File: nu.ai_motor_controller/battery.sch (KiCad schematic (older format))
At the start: 42 parts, among them J12 XT60_RA_MALE, J13 S4B-XH-A, J14 NP_Screw_Terminal_01x02, J15 XT60_RA_MALE, J16 S4B-XH-A, J17 S4B-XH-A, J18 XT60_RA_FEMALE, Q1 IRF9540N, Q2 SSM3K35AMFV, Q4 SSM3K35AMFV, SW2 TACTILE_SWITCH, SW3 TACTILE_SWITCH

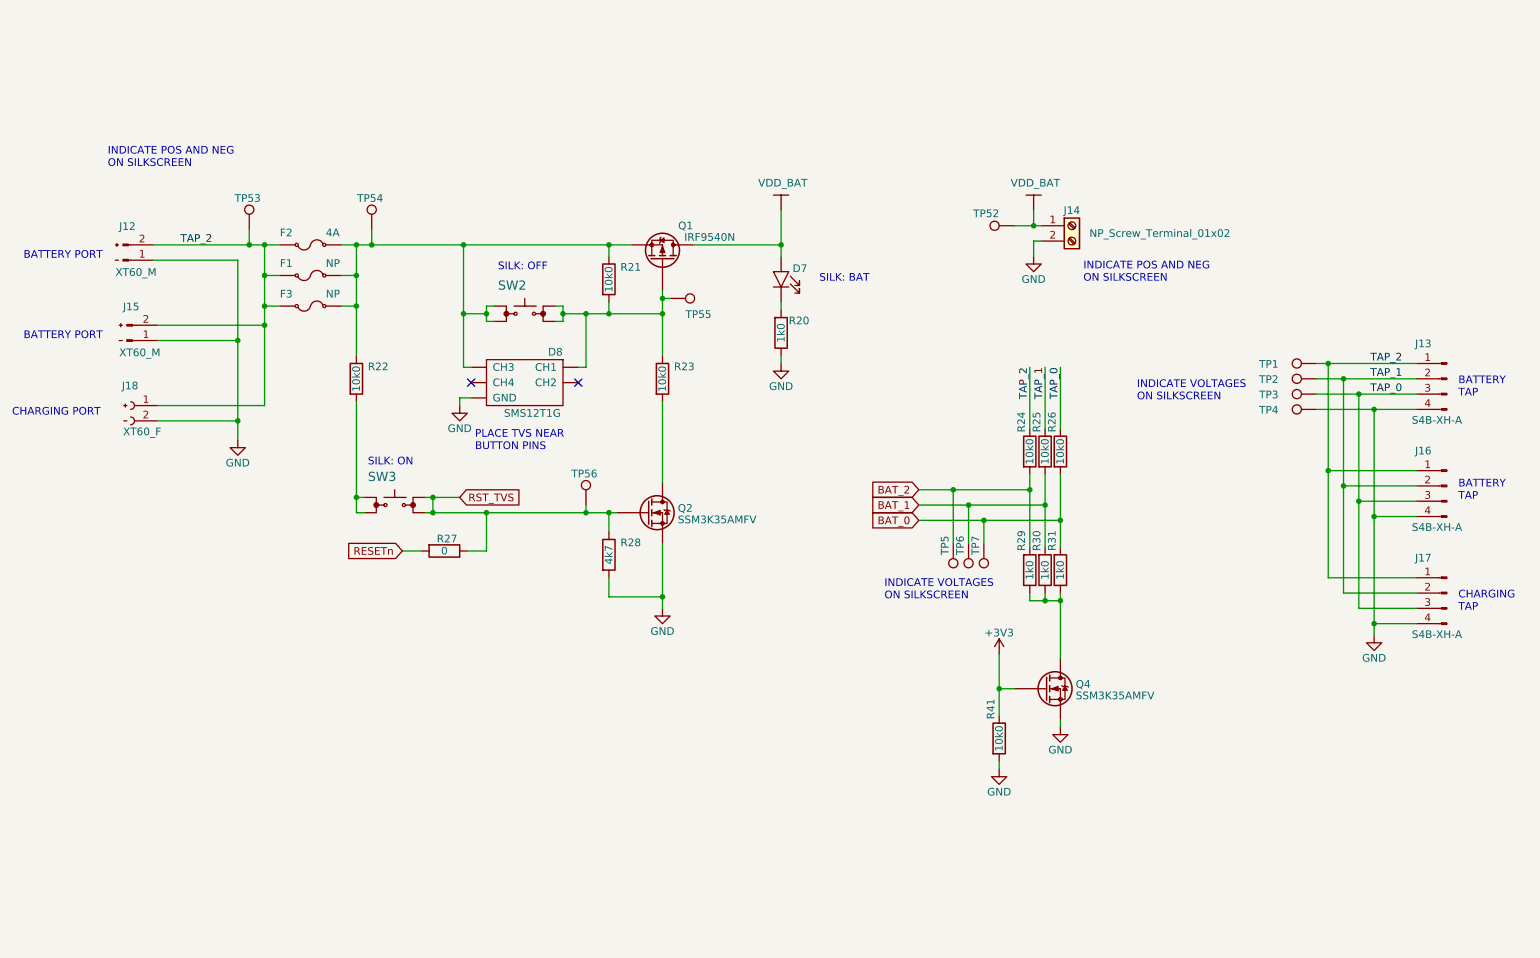
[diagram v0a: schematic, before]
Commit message: automated commit
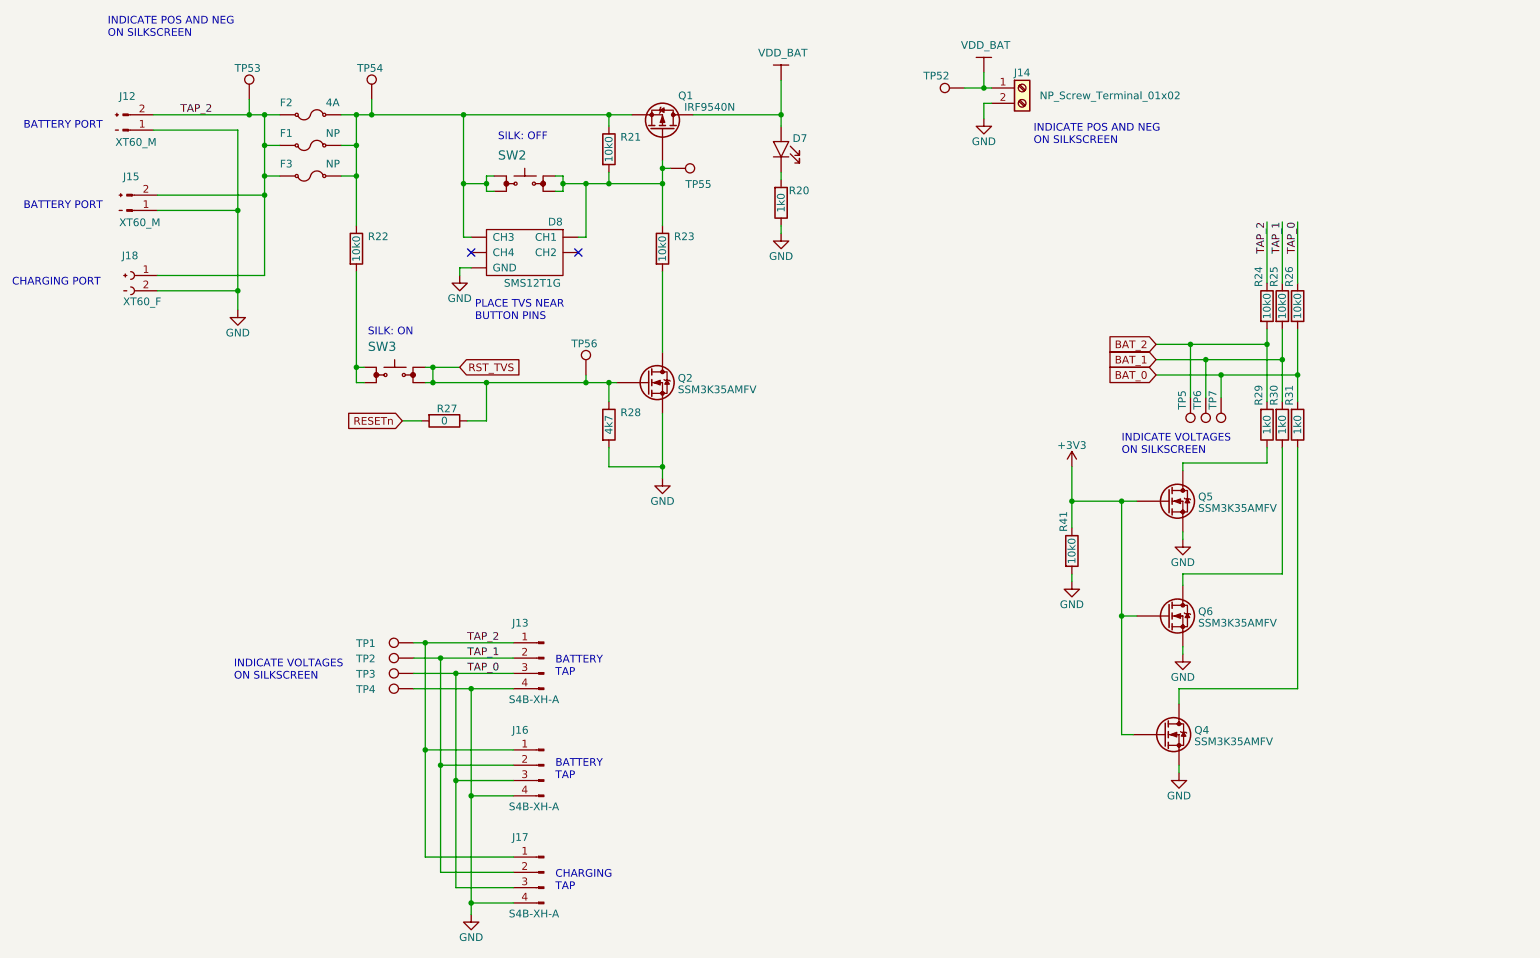
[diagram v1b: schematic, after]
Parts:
- added Q5, Q6: SSM3K35AMFV, Package_TO_SOT_SMD:SOT-723, symbol custom:SSM3K35AMFV
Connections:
- net +3V3: now also Q5.1 (G), Q6.1 (G)
- net GND: now also Q5.2 (S), Q6.2 (S)
- net at Q4.3 (D), R31.2: no longer R29.2, R30.2
- new net: Q5.3 (D), R29.2
- new net: Q6.3 (D), R30.2
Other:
- note removed: "SILK: BAT"
- moved on the sheet: D7, D8, F1, F2, F3, J12, J13, J14, J15, J16, J17, J18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
